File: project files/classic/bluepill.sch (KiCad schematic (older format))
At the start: 38 parts, among them J1 USB_B_Micro, J2 Boot, J3 Left Row, J4 Right Row, J5 SWD, SW1 Reset, U1 RT8183-33, U2 STM32F103C8Tx, Y1 8MHz, Y2 32768Hz

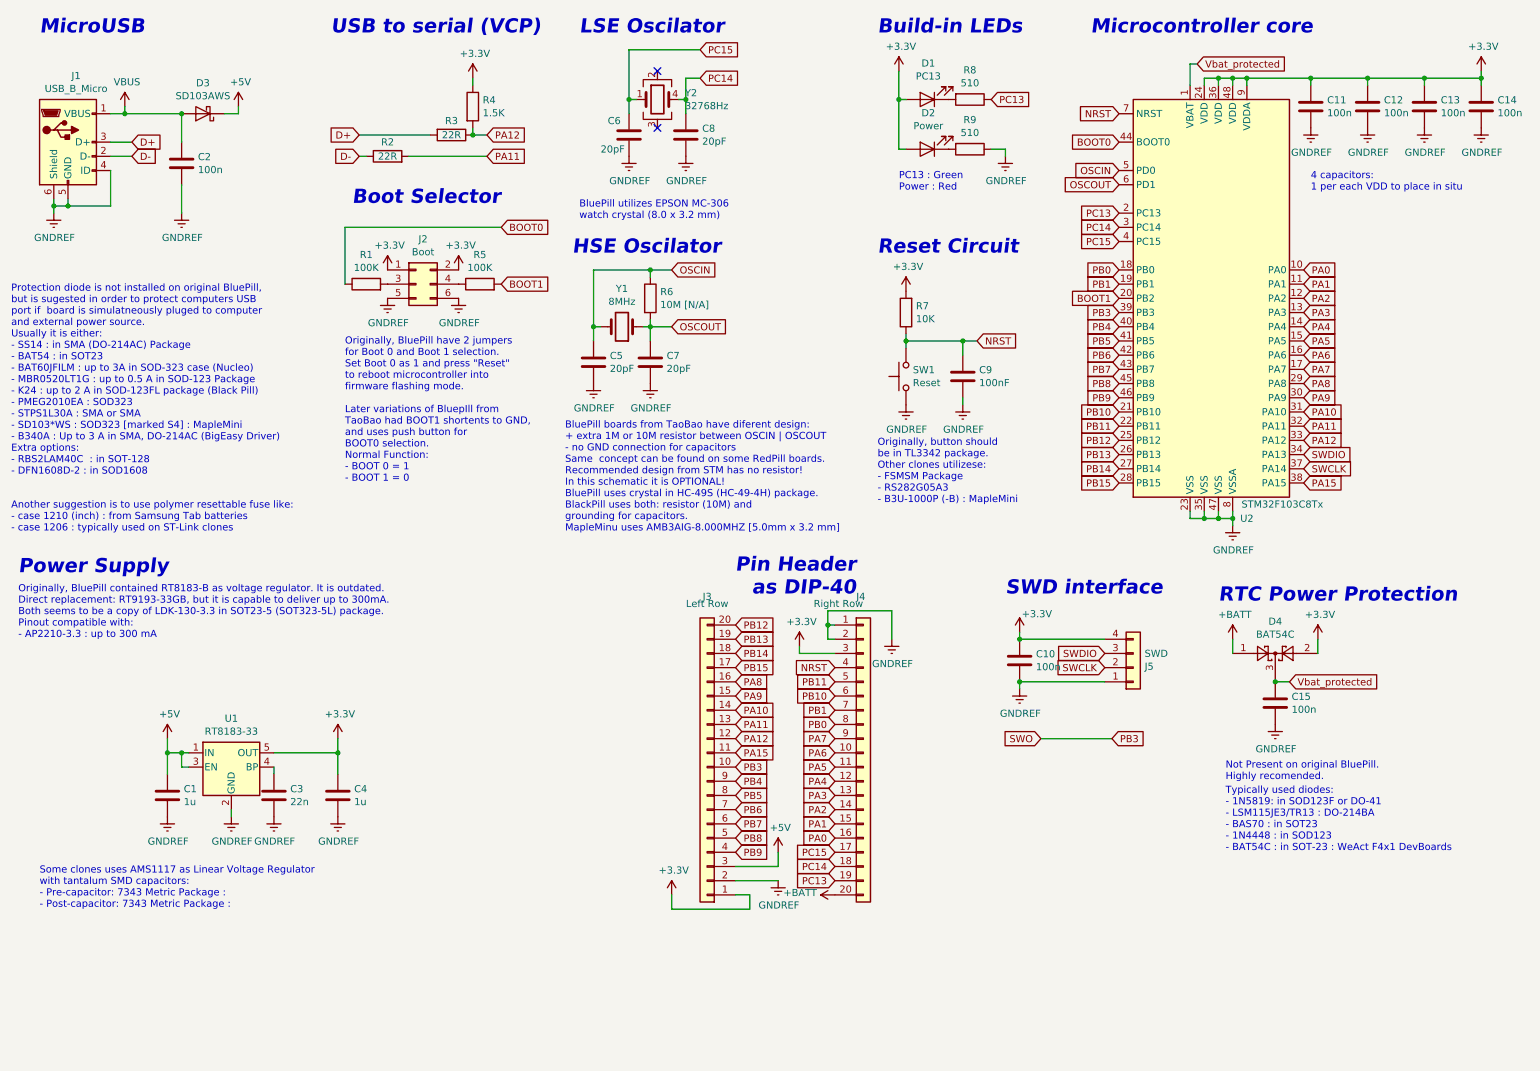
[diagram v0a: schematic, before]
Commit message: Updates
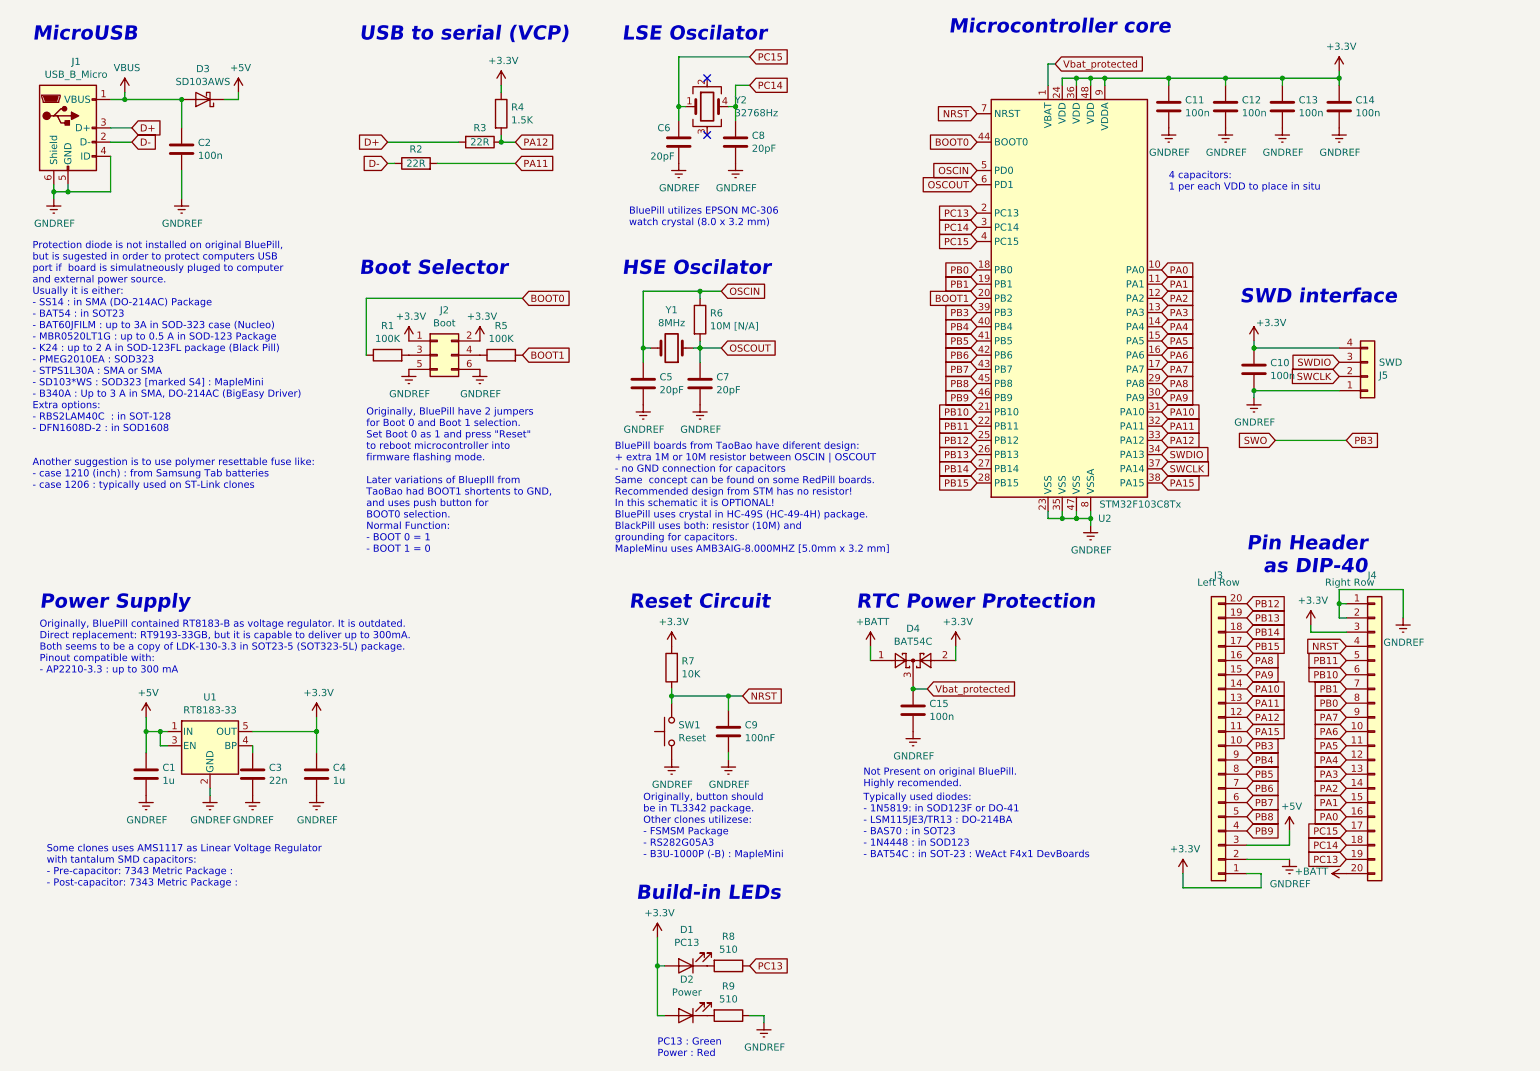
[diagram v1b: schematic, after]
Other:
- moved on the sheet: C1, C10, C11, C12, C13, C14, C15, C2, C3, C4, C5, C6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
